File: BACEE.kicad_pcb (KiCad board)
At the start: 2 copper layers, 42.7 x 29 mm, 17 parts, among them J1 Serial, J2 Digital pins, J3 ICSP, J4 I2C, U1 24LC1025, U2 24LC1025, U3 DS1337_KTH, U4 ATMEGA328P-AU, Y1 Crystal 32MHz, Y2 Crystal 16MHz

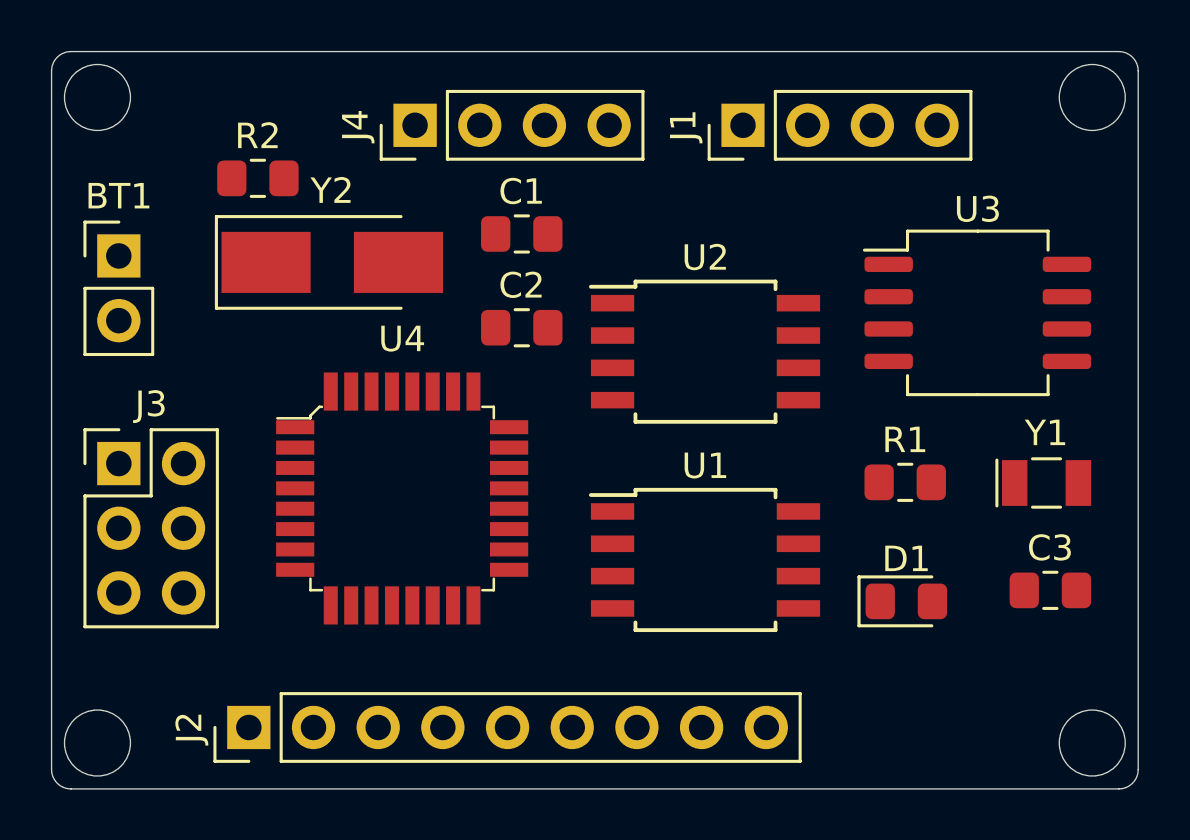
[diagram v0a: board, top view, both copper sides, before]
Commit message: routed using 4 layers
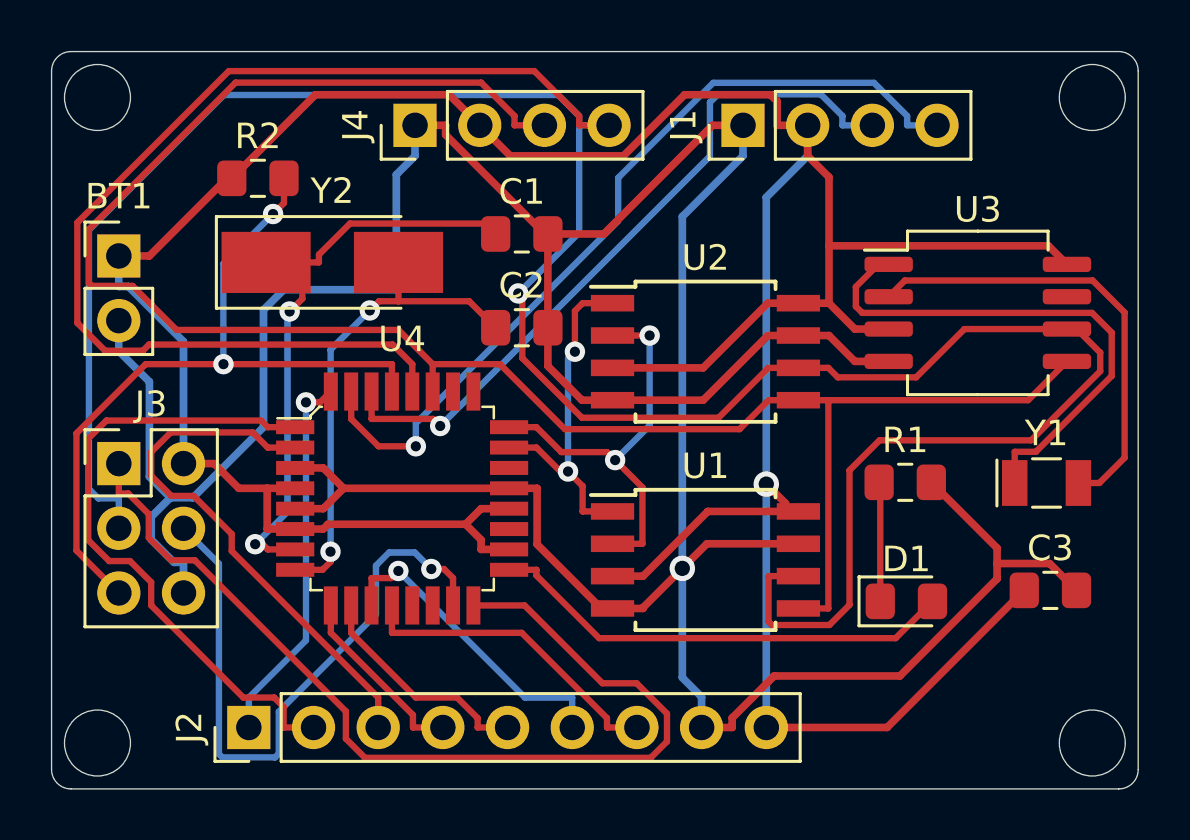
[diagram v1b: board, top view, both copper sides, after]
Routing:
- net GND: track 0.00 -> 145.8 mm, vias 0 -> 1
- net SCK: track 0.00 -> 139.5 mm, vias 0 -> 1
- net VCC: track 0.00 -> 136.4 mm, vias 0 -> 1
- net SDA: track 0.00 -> 75.6 mm
- net MISO: track 0.00 -> 38.9 mm
- net TX: track 0.00 -> 32.9 mm, vias 0 -> 1
- net RST: track 0.00 -> 29.8 mm, vias 0 -> 2
- net RX: track 0.00 -> 28.2 mm, vias 0 -> 1
- net MOSI: track 0.00 -> 25.6 mm, vias 0 -> 1
- net D3: track 0.00 -> 25.4 mm
- net Net-(C1-Pad1): track 0.00 -> 23.5 mm, vias 0 -> 2
- net D4: track 0.00 -> 21.2 mm
- net Net-(U3-Pad1): track 0.00 -> 20.9 mm
- net Net-(C2-Pad1): track 0.00 -> 19.1 mm, vias 0 -> 2
- net Net-(D1-Pad2): track 0.00 -> 18.5 mm
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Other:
- copper layers 2 -> 4

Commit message: silk screen added
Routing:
- added copper zone on In2.Cu, net GND
